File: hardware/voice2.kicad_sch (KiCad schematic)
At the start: 29 parts, among them IC1 LM13700, U12 MCP4922-E/P, U13 SSM2044

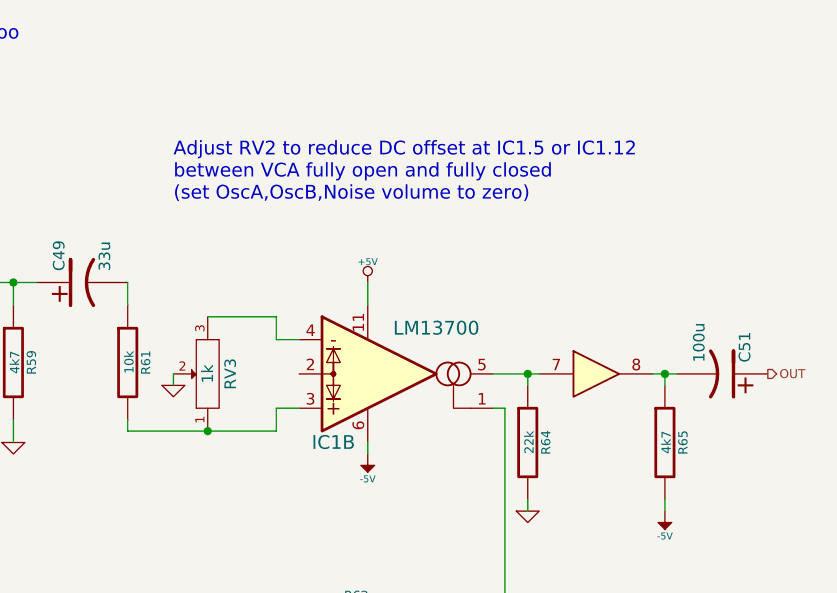
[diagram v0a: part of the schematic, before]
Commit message: hardware: OverCycler3 schematics WIP
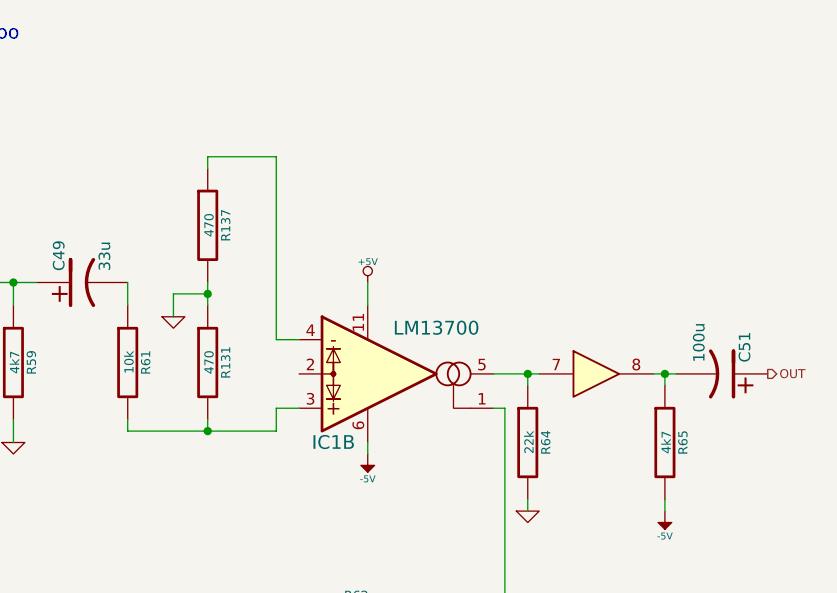
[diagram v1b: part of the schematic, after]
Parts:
- removed RV3: 1k, ~, symbol overcycler2-rescue:POT
- added R131, R137: 470, ~, symbol overcycler2-rescue:R
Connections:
- net GND: now also R131.1, R137.2
- net at IC1.3 (+), R61.2: now also R131.2
- net at IC1.4 (-): now also R137.1
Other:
- note removed: "Adjust RV2 to reduce DC offset at IC1.5 or IC1.12 between VCA fully open and fully closed (set OscA,OscB,Noise volume to zero)"

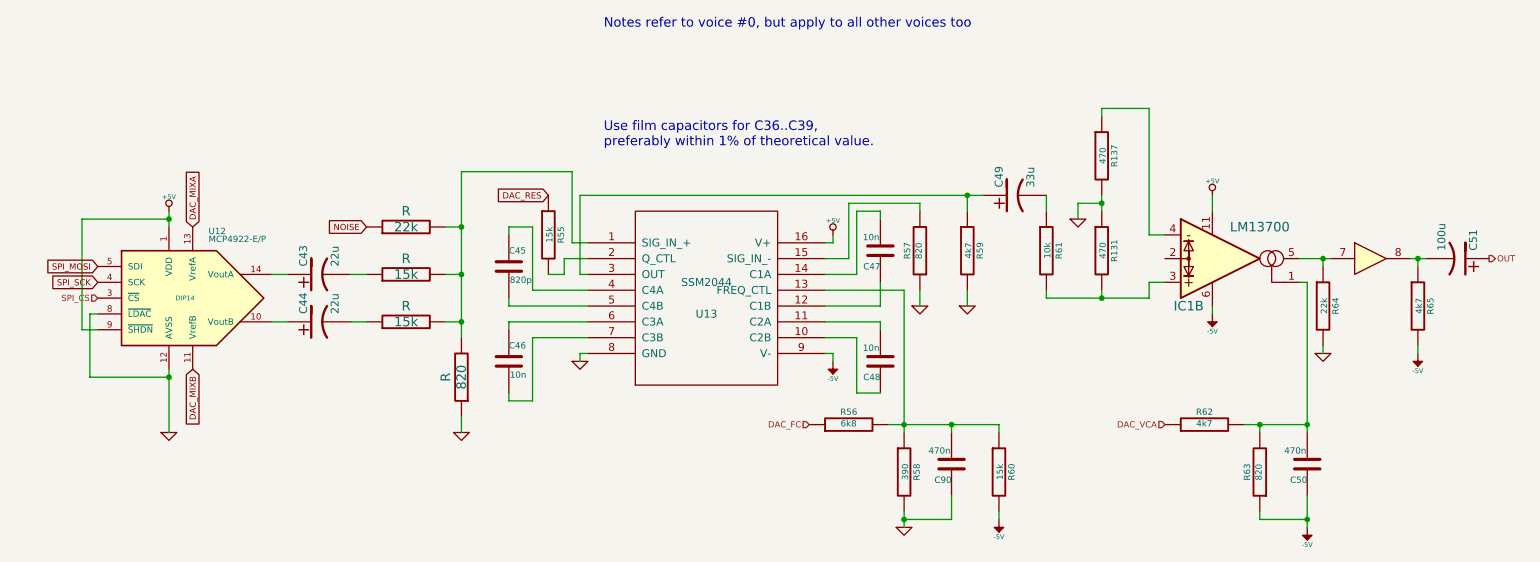
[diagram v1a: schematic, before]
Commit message: hardware: OverCycler3 schematics WIP2
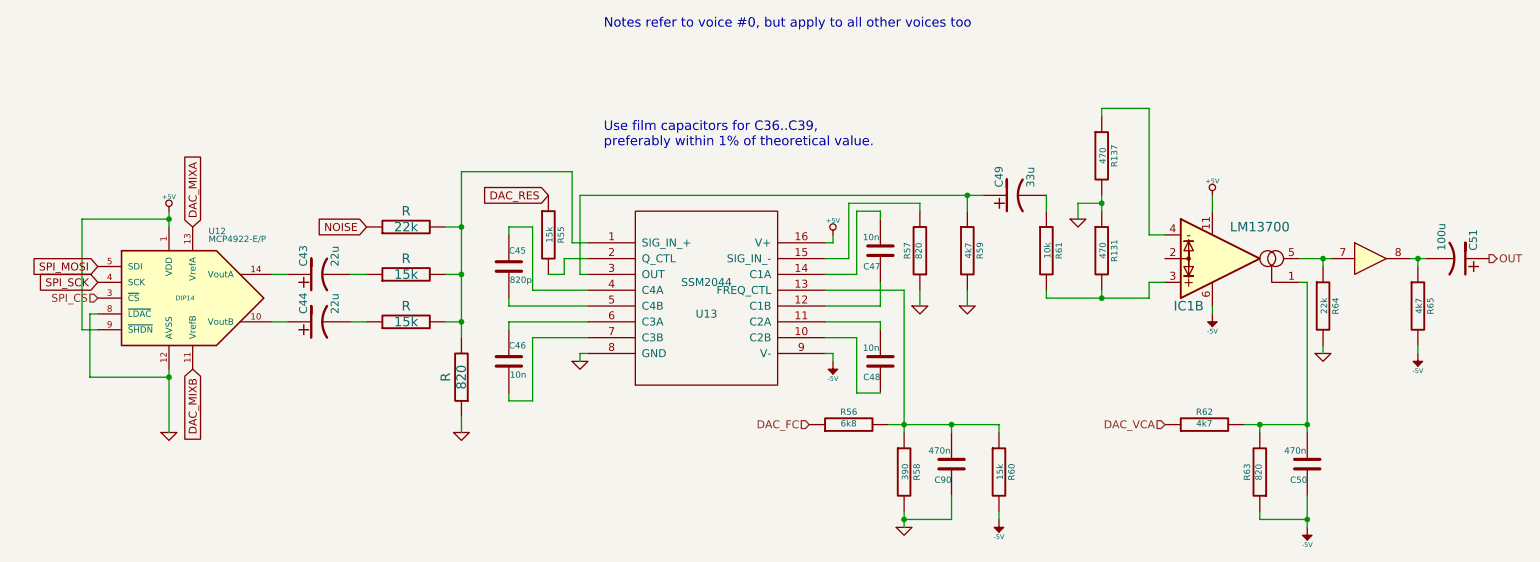
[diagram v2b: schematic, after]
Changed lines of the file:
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@@
   )
   (global_label "SPI_MOSI" (shape input) (at 35.56 90.17 180)
-    (effects (font (size 0.9906 0.9906)) (justify right))
+    (effects (font (size 1.27 1.27)) (justify right))
     (property "Intersheetrefs" "${INTERSHEET_REFS}" (at 35.56 90.17 0)
       (effects (font (size 1.27 1.27)) hide)
@@
   )
   (global_label "NOISE" (shape input) (at 78.74 83.82 180)
-    (effects (font (size 0.9906 0.9906)) (justify right))
+    (effects (font (size 1.27 1.27)) (justify right))
     (property "Intersheetrefs" "${INTERSHEET_REFS}" (at 78.74 83.82 0)
       (effects (font (size 1.27 1.27)) hide)
@@
   )
   (global_label "SPI_SCK" (shape input) (at 35.56 92.71 180)
-    (effects (font (size 0.9906 0.9906)) (justify right))
+    (effects (font (size 1.27 1.27)) (justify right))
     (property "Intersheetrefs" "${INTERSHEET_REFS}" (at 35.56 92.71 0)
       (effects (font (size 1.27 1.27)) hide)
@@
   )
   (global_label "DAC_RES" (shape input) (at 107.95 78.74 180)
-    (effects (font (size 0.9906 0.9906)) (justify right))
+    (effects (font (size 1.27 1.27)) (justify right))
     (property "Intersheetrefs" "${INTERSHEET_REFS}" (at 107.95 78.74 0)
       (effects (font (size 1.27 1.27)) hide)
@@
   )
   (global_label "DAC_MIXA" (shape input) (at 50.8 83.82 90)
-    (effects (font (size 0.9906 0.9906)) (justify left))
+    (effects (font (size 1.27 1.27)) (justify left))
     (property "Intersheetrefs" "${INTERSHEET_REFS}" (at 50.8 83.82 0)
       (effects (font (size 1.27 1.27)) hide)
@@
   )
   (global_label "DAC_MIXB" (shape input) (at 50.8 106.68 270)
-    (effects (font (size 0.9906 0.9906)) (justify right))
+    (effects (font (size 1.27 1.27)) (justify right))
     (property "Intersheetrefs" "${INTERSHEET_REFS}" (at 50.8 106.68 0)
       (effects (font (size 1.27 1.27)) hide)
@@
   )
   (hierarchical_label "OUT" (shape output) (at 259.08 88.9 0) (fields_autoplaced)
-    (effects (font (size 0.9906 0.9906)) (justify left))
+    (effects (font (size 1.27 1.27)) (justify left))
   )
   (hierarchical_label "DAC_FC" (shape input) (at 149.86 115.57 180) (fields_autoplaced)
-    (effects (font (size 0.9906 0.9906)) (justify right))
+    (effects (font (size 1.27 1.27)) (justify right))
   )
   (hierarchical_label "DAC_VCA" (shape input) (at 207.01 115.57 180) (fields_autoplaced)
-    (effects (font (size 0.9906 0.9906)) (justify right))
+    (effects (font (size 1.27 1.27)) (justify right))
   )
   (hierarchical_label "SPI_CS" (shape input) (at 35.56 95.25 180) (fields_autoplaced)
-    (effects (font (size 0.9906 0.9906)) (justify right))
+    (effects (font (size 1.27 1.27)) (justify right))
   )
   (symbol (lib_id "overcycler2-rescue:SSM2044") (at 133.35 95.25 0) (unit 1)
